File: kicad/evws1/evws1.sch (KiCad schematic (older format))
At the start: 66 parts, among them J1 Screw_Terminal_01x03, J10 Screw_Terminal_01x04, J2 Screw_Terminal_01x02, J3 HB9500-2P, J4 HB9500-3P, J5 Screw_Terminal_01x04, J6 Screw_Terminal_01x03, J7 Screw_Terminal_01x02, J8 HB9500-2P, J9 HB9500-3P, K1 G3MB-202P, K2 G3MB-202P, M1 HLK-PM01, M2 dc-dc-buck-converter-5v-to-3.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, M3 dc-dc-converter-5v-to-p12v-m1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, Q1 AO3401, Q2 AO3401, SW1 SW_SS13F06-G5, SW2 SW_SS13F06-G5, T1 ZMPT101B, T2 ZMPT101B, U2 ACS712-30, U3 ACS712-30

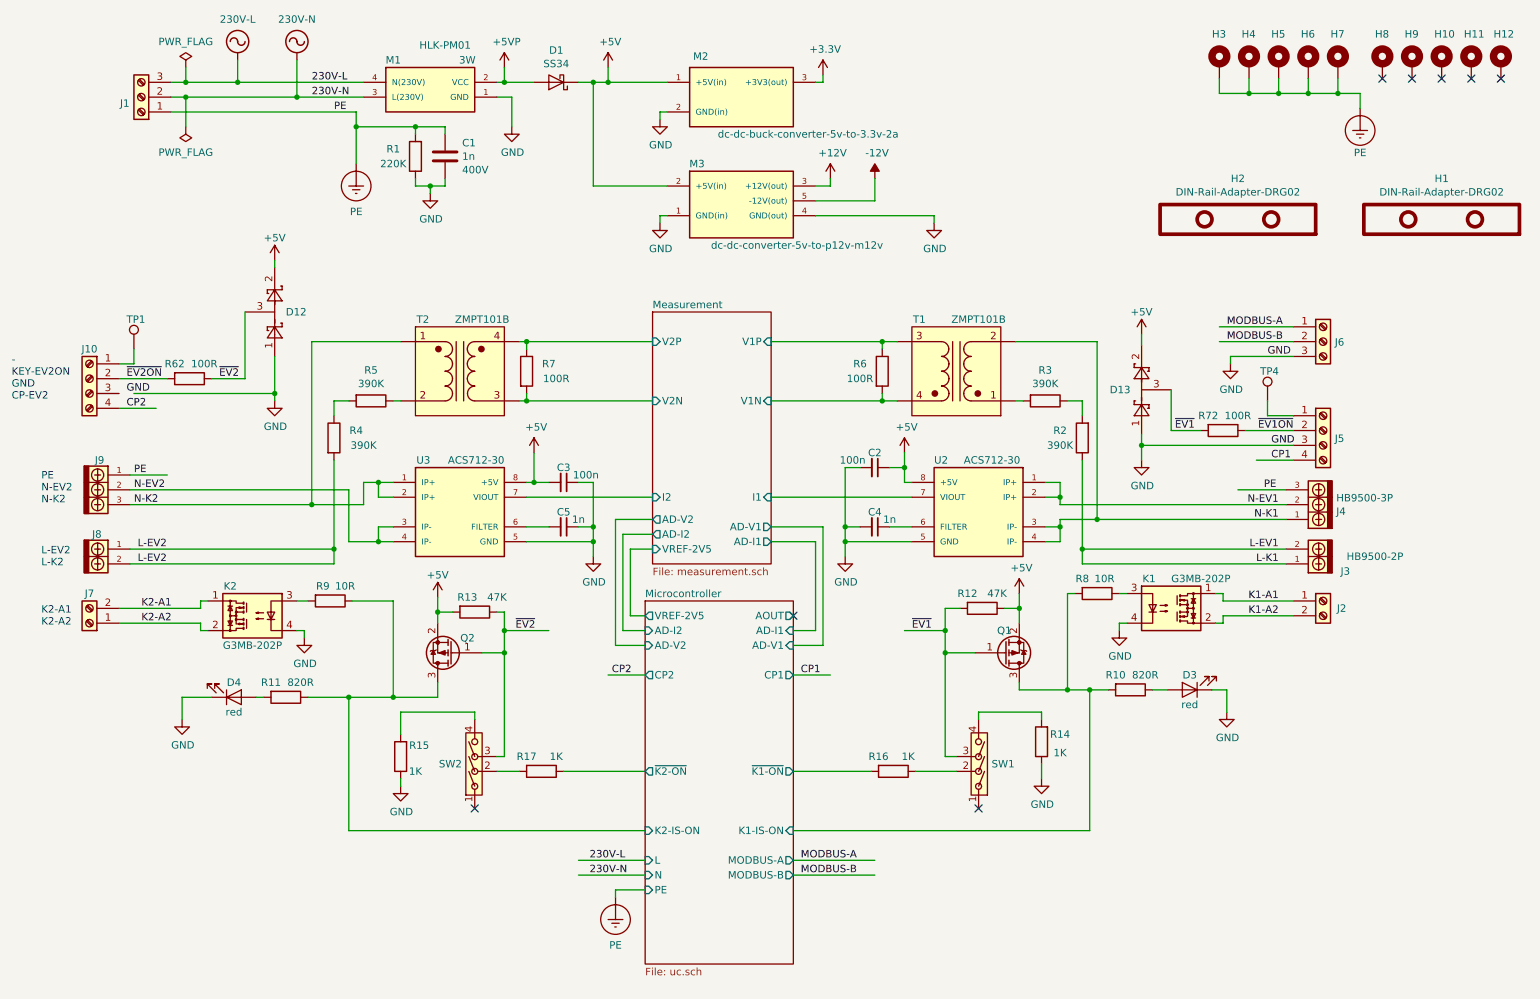
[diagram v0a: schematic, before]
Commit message: ...
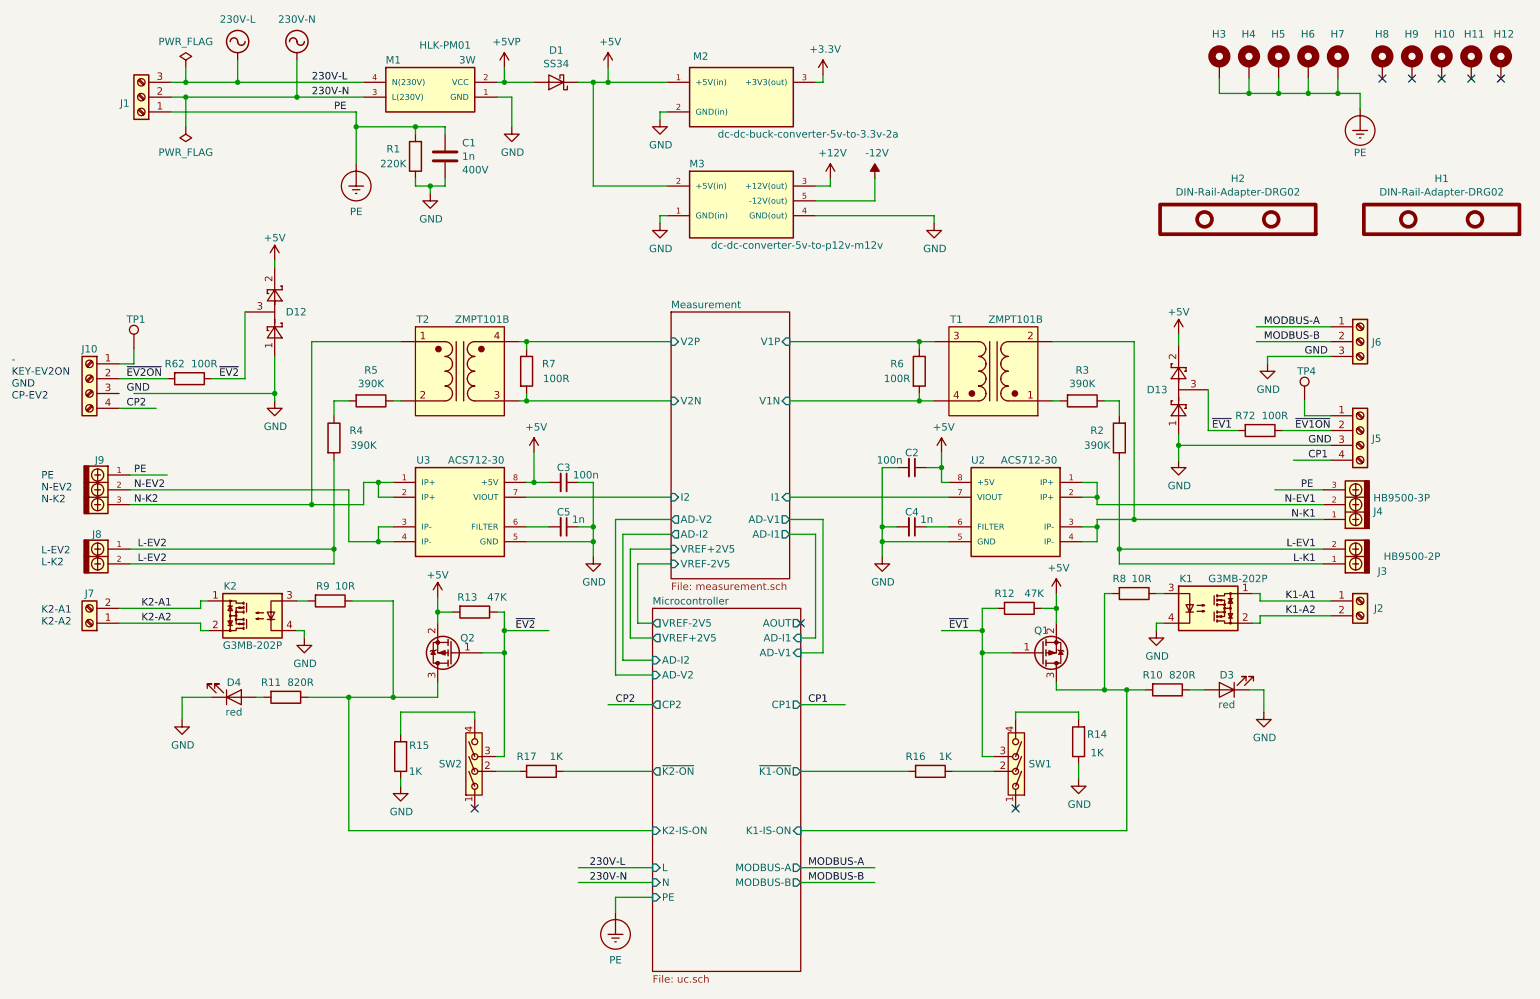
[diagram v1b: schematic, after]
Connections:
- wire segments 254 -> 257
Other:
- moved on the sheet: C2, C4, D13, D3, J2, J3, J4, J5, J6, K1, Q1, R10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
